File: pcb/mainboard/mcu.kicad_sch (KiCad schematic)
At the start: 24 parts, among them SW701 EVQPUJ02K, U701 W25Q32JV, U702 RP2040, Y701 12MHz

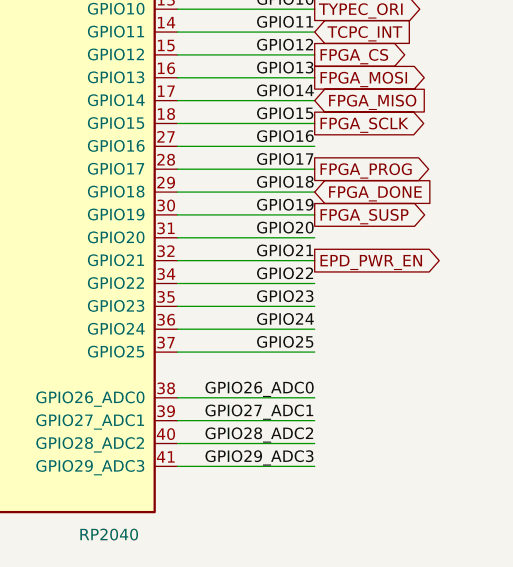
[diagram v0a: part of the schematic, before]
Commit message: pcb: r0p6
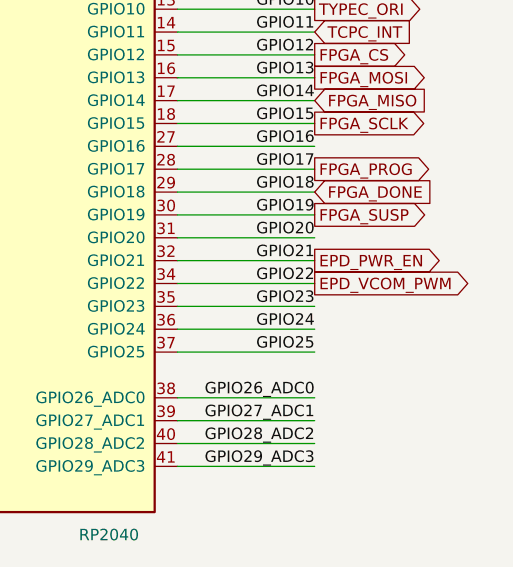
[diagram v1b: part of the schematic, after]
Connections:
- net GPIO22 renamed EPD_VCOM_PWM

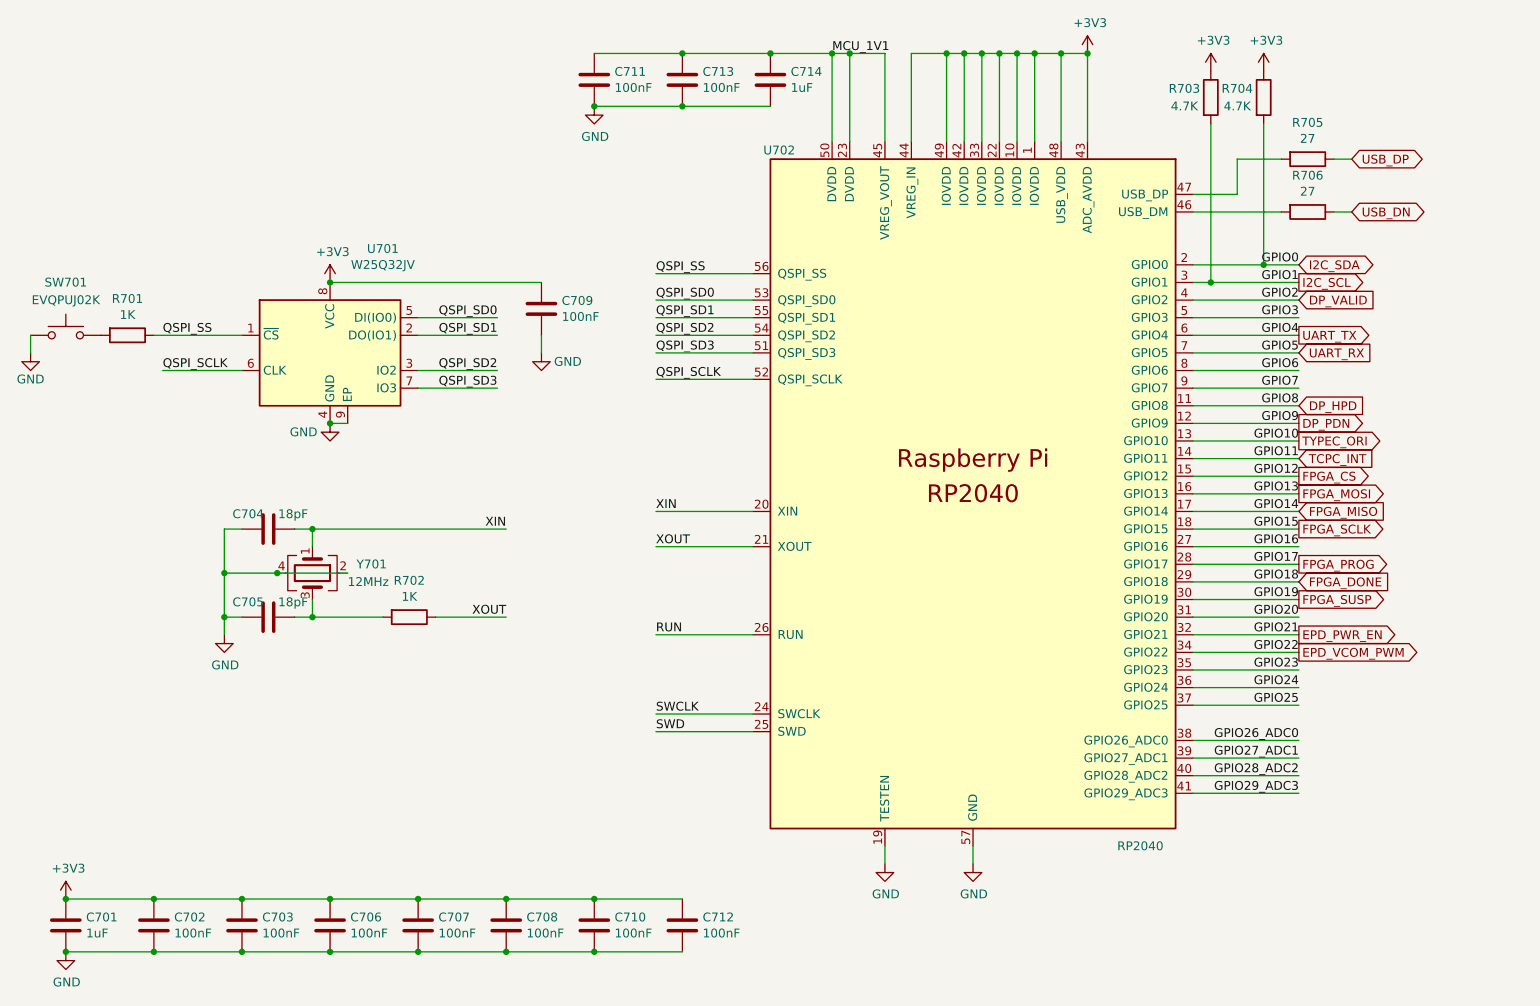
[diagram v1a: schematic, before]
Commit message: r0p7 wip, check in before switch to kicad 8
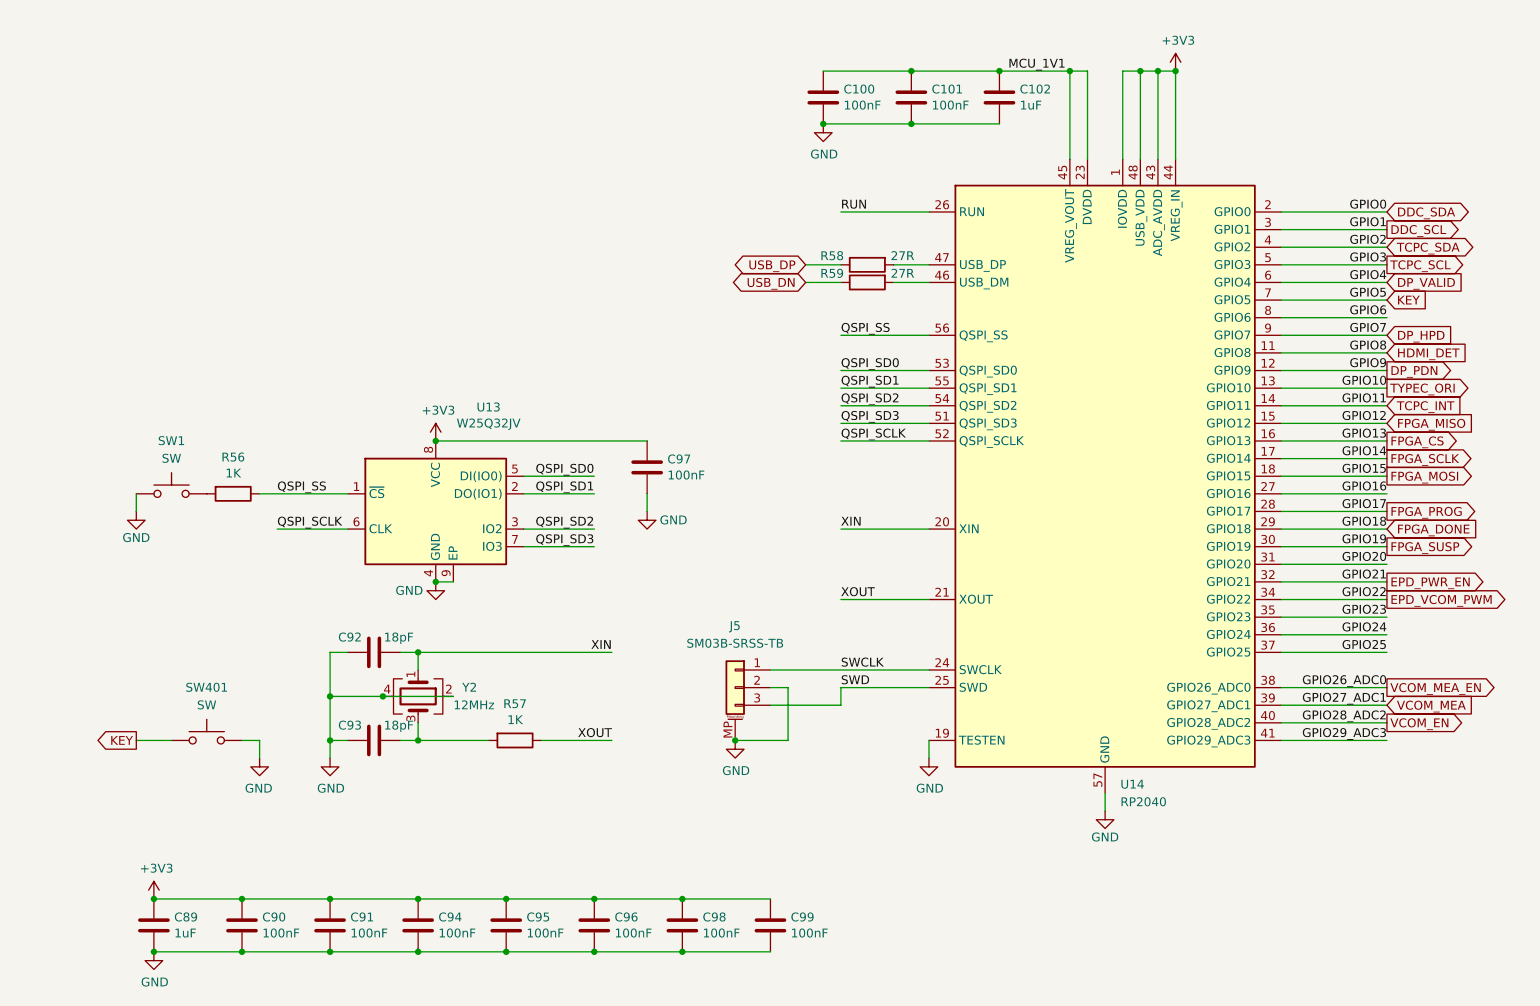
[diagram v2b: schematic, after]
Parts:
- removed R703, R704: 4.7K, Resistor_SMD:R_0402_1005Metric, symbol Device:R
- removed U702: RP2040, footprints:RP2040-QFN-56, symbol MCU_RaspberryPi_RP2040:RP2040
- added J5: SM03B-SRSS-TB, Connector_JST:JST_SH_SM03B-SRSS-TB_1x03-1MP_P1.00mm_Horizontal, symbol Connector_Generic_MountingPin:Conn_01x03_MountingPin
- added SW401: SW, Button_Switch_SMD:Panasonic_EVQPUL_EVQPUC, symbol Switch:SW_Push
- added U14: RP2040, footprints:RP2040-QFN-56, symbol MCU_RaspberryPi:RP2040
- R58: renamed from R705; value 27 -> 27R
- R59: renamed from R706; value 27 -> 27R
- SW1: renamed from SW701; value EVQPUJ02K -> SW; footprint Button_Switch_SMD:SW_SPST_CK_KXT3 -> Button_Switch_SMD:Panasonic_EVQPUL_EVQPUC
- renumbered C711 to C100, C713 to C101, C714 to C102, C701 to C89, C702 to C90, C703 to C91, C704 to C92, C705 to C93, C706 to C94, C707 to C95, C708 to C96, C709 to C97, C710 to C98, C712 to C99, R701 to R56, R702 to R57, U701 to U13, Y701 to Y2
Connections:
- net +3V3: now also U14.1 (IOVDD), U14.10 (IOVDD), U14.22 (IOVDD), U14.33 (IOVDD), U14.42 (IOVDD), U14.43 (ADC_AVDD), U14.44 (VREG_IN), U14.48 (USB_VDD), U14.49 (IOVDD)
- net DP_HPD: now also U14.9 (GPIO7)
- net DP_PDN: now also U14.12 (GPIO9)
- net DP_VALID: now also U14.6 (GPIO4)
- net EPD_PWR_EN: now also U14.32 (GPIO21)
- net EPD_VCOM_PWM: now also U14.34 (GPIO22)
- net FPGA_CS: now also U14.16 (GPIO13)
- net FPGA_DONE: now also U14.29 (GPIO18)
- net FPGA_MISO: now also U14.15 (GPIO12)
- net FPGA_MOSI: now also U14.18 (GPIO15)
- net FPGA_PROG: now also U14.28 (GPIO17)
- net FPGA_SCLK: now also U14.17 (GPIO14)
- net FPGA_SUSP: now also U14.30 (GPIO19)
- net GND: now also J5.2 (Pin_2), J5.MP (MountPin), SW401.2, U14.19 (TESTEN), U14.57 (GND)
- net GPIO16: now also U14.27 (GPIO16)
- net GPIO20: now also U14.31 (GPIO20)
- net GPIO23: now also U14.35 (GPIO23)
- net GPIO24: now also U14.36 (GPIO24)
- net GPIO25: now also U14.37 (GPIO25)
- net GPIO29_ADC3: now also U14.41 (GPIO29_ADC3)
- net GPIO6: now also U14.8 (GPIO6)
- net MCU_1V1: now also U14.23 (DVDD), U14.45 (VREG_VOUT), U14.50 (DVDD)
- net QSPI_SCLK: now also U14.52 (QSPI_SCLK)
- net QSPI_SD0: now also U14.53 (QSPI_SD0)
- net QSPI_SD1: now also U14.55 (QSPI_SD1)
- net QSPI_SD2: now also U14.54 (QSPI_SD2)
- net QSPI_SD3: now also U14.51 (QSPI_SD3)
- net QSPI_SS: now also U14.56 (QSPI_SS)
- net RUN: now also U14.26 (RUN)
- net SWCLK: now also J5.1 (Pin_1), U14.24 (SWCLK)
- net SWD: now also J5.3 (Pin_3), U14.25 (SWD)
- net TCPC_INT: now also U14.14 (GPIO11)
- net TYPEC_ORI: now also U14.13 (GPIO10)
- net XIN: now also U14.20 (XIN)
- net XOUT: now also U14.21 (XOUT)
- net at R59.2: now also U14.46 (USB_DM)
- net at R58.2: now also U14.47 (USB_DP)
- new net DDC_SCL: U14.3 (GPIO1)
- new net DDC_SDA: U14.2 (GPIO0)
- new net HDMI_DET: U14.11 (GPIO8)
- new net KEY: SW401.1, U14.7 (GPIO5)
- new net TCPC_SCL: U14.5 (GPIO3)
- new net TCPC_SDA: U14.4 (GPIO2)
- new net VCOM_EN: U14.40 (GPIO28_ADC2)
- new net VCOM_MEA: U14.39 (GPIO27_ADC1)
- new net VCOM_MEA_EN: U14.38 (GPIO26_ADC0)
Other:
- moved on the sheet: C100, C101, C102, C89, C90, C91, C92, C93, C94, C95, C96, C97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
